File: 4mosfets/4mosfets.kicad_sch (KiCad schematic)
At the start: 22 parts, among them J1 Conn_01x04_Pin, J2 Conn_01x02_Pin, J3 Conn_01x02_Pin, J4 Conn_01x02_Pin, J5 Conn_01x02_Pin, J6 Conn_01x02_Pin, Q1 AO3400A, Q2 AO3400A, Q3 AO3400A, Q4 AO3400A

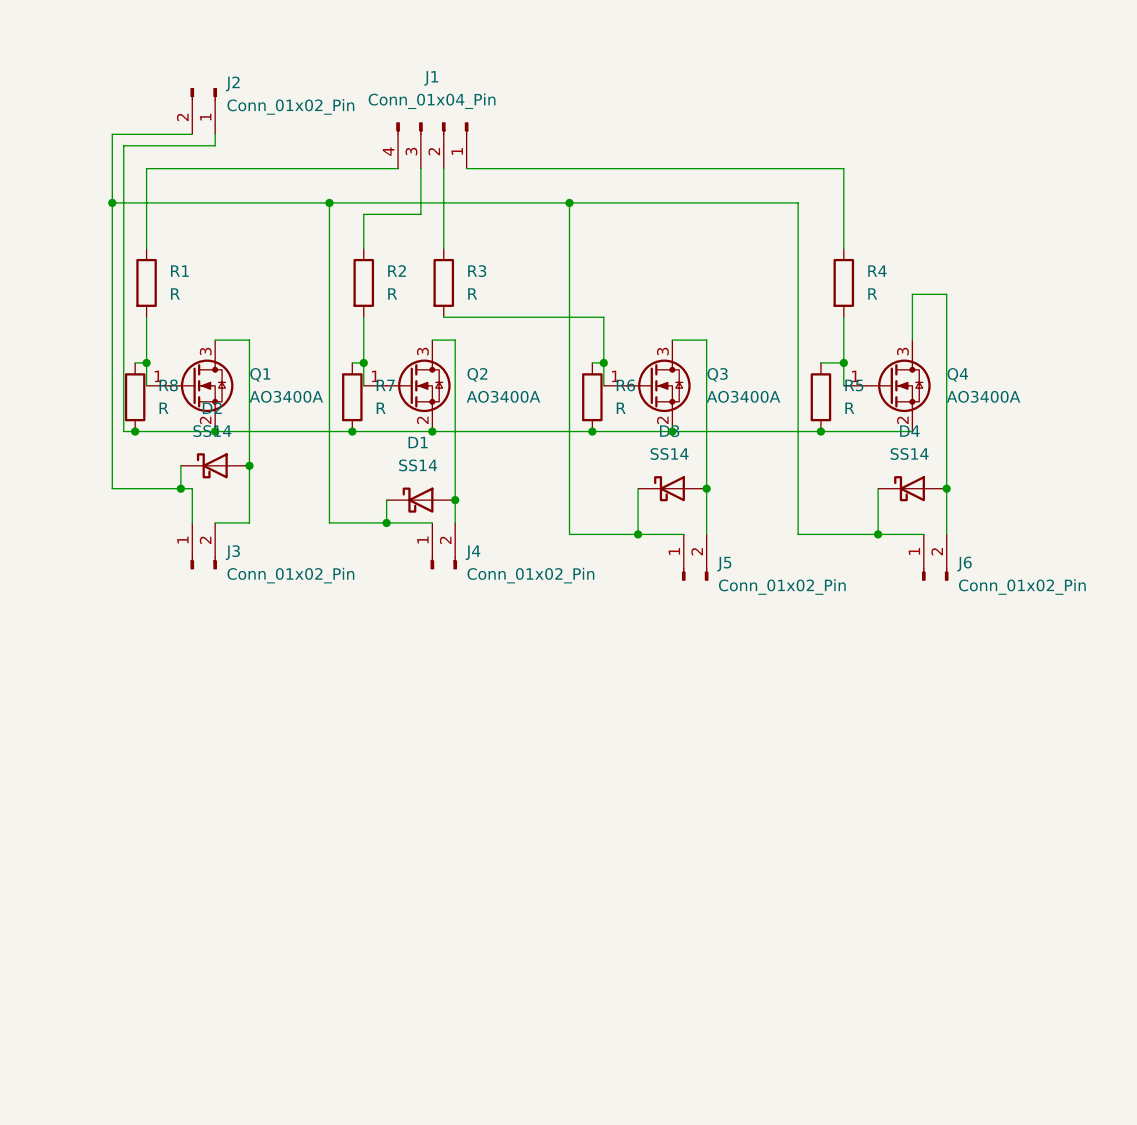
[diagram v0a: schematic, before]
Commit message: updated pcb
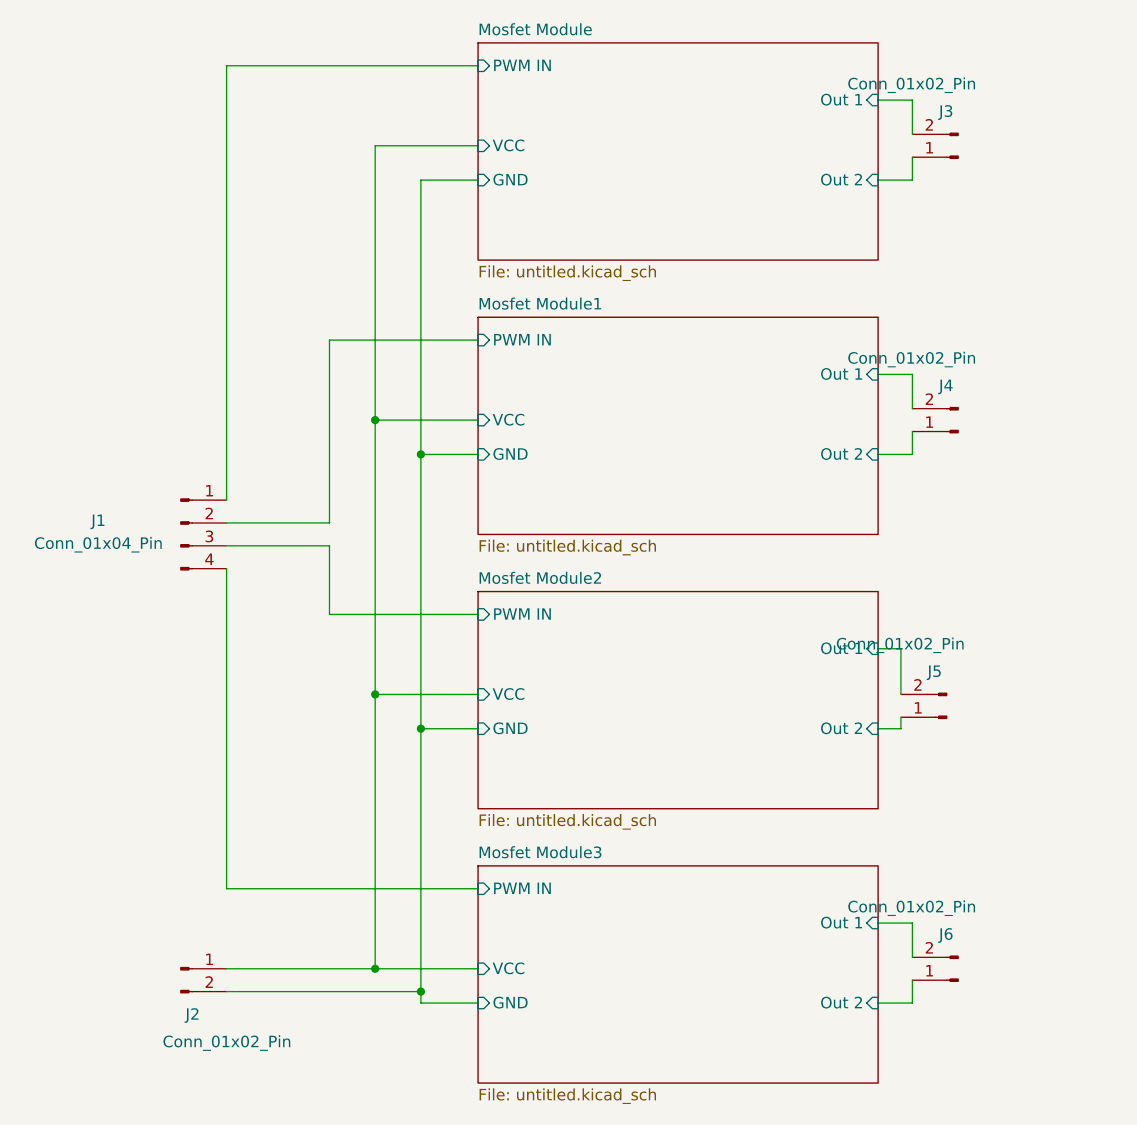
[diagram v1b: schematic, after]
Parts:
- removed D1, D2, D3, D4: SS14, Diode_SMD:D_SMA, symbol Diode:SS14
- removed Q1, Q2, Q3, Q4: AO3400A, Package_TO_SOT_SMD:SOT-23, symbol Transistor_FET:AO3400A
- removed R1, R2, R3, R4, R5, R6, R7, R8: R, Resistor_SMD:R_0805_2012Metric, symbol Device:R
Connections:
- net Mosfet Module/VCC: now reaches J2.1 (Pin_1)
- net Mosfet Module1/Out 1: now reaches J4.2 (Pin_2)
- net Mosfet Module2/Out 1: now reaches J5.2 (Pin_2)
- net Mosfet Module3/Out 1: now reaches J6.2 (Pin_2)
- net Mosfet Module/Out 1: now reaches J3.2 (Pin_2)
- net Mosfet Module2/PWM IN: now reaches J1.3 (Pin_3)
- net Mosfet Module3/PWM IN: now reaches J1.4 (Pin_4)
- net Mosfet Module/PWM IN: now reaches J1.1 (Pin_1)
- net Mosfet Module1/PWM IN: now reaches J1.2 (Pin_2)
- new net Mosfet Module/GND: J2.2 (Pin_2)
- new net Mosfet Module/Out 2: J3.1 (Pin_1)
- new net Mosfet Module1/Out 2: J4.1 (Pin_1)
- new net Mosfet Module2/Out 2: J5.1 (Pin_1)
- new net Mosfet Module3/Out 2: J6.1 (Pin_1)
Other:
- added sheet Mosfet Module (untitled.kicad_sch)
- added sheet Mosfet Module1 (untitled.kicad_sch)
- added sheet Mosfet Module2 (untitled.kicad_sch)
- added sheet Mosfet Module3 (untitled.kicad_sch)
- moved on the sheet: J1, J2
